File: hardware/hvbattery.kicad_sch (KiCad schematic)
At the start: 0 parts

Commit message: initial review again
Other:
- added sheet HV -> 12V (HV_converter.kicad_sch)
- added sheet HV Input (HV_protection.kicad_sch)
- note added: "HV input protection + sensing"
- note added: "HV vicor + sensing"

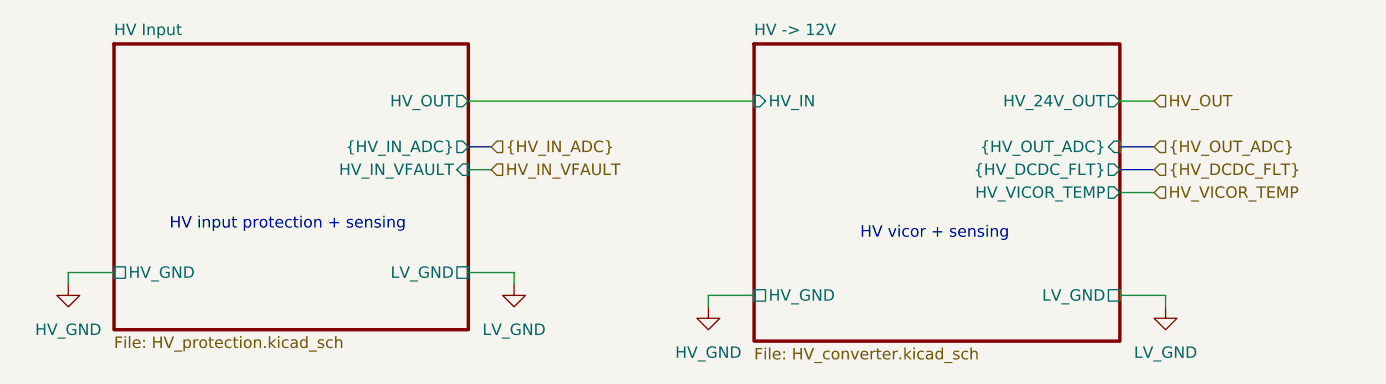
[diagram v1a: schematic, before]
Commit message: progress!
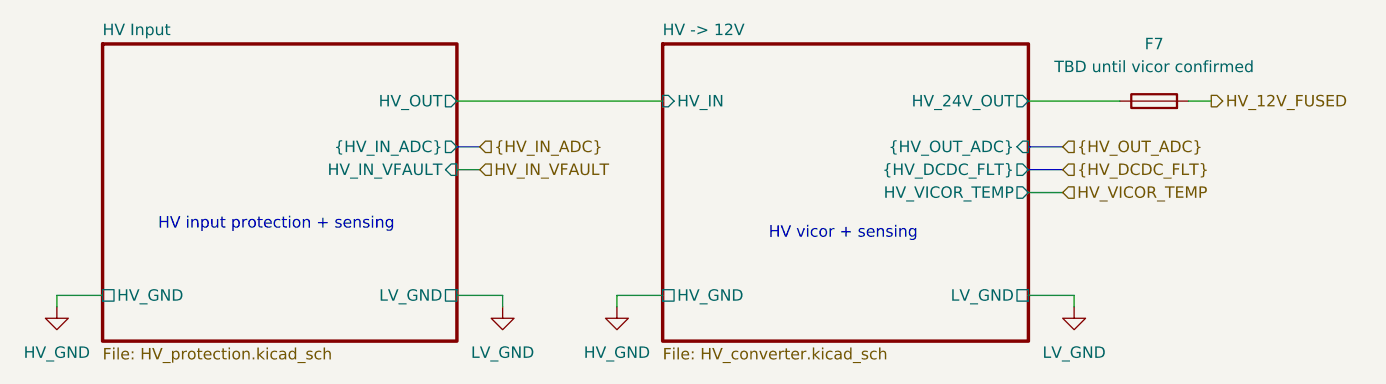
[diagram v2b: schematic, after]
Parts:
- added F7: TBD until vicor confirmed, LHRS_Power:Fuse-3557-2, symbol Device:Fuse
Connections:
- new net HV -> 12V/HV_24V_OUT: F7.1
- new net HV_12V_FUSED: F7.2
